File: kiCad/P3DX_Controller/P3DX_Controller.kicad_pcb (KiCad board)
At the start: 2 copper layers, 2 parts, among them U1 ESP32-WROOM-32E

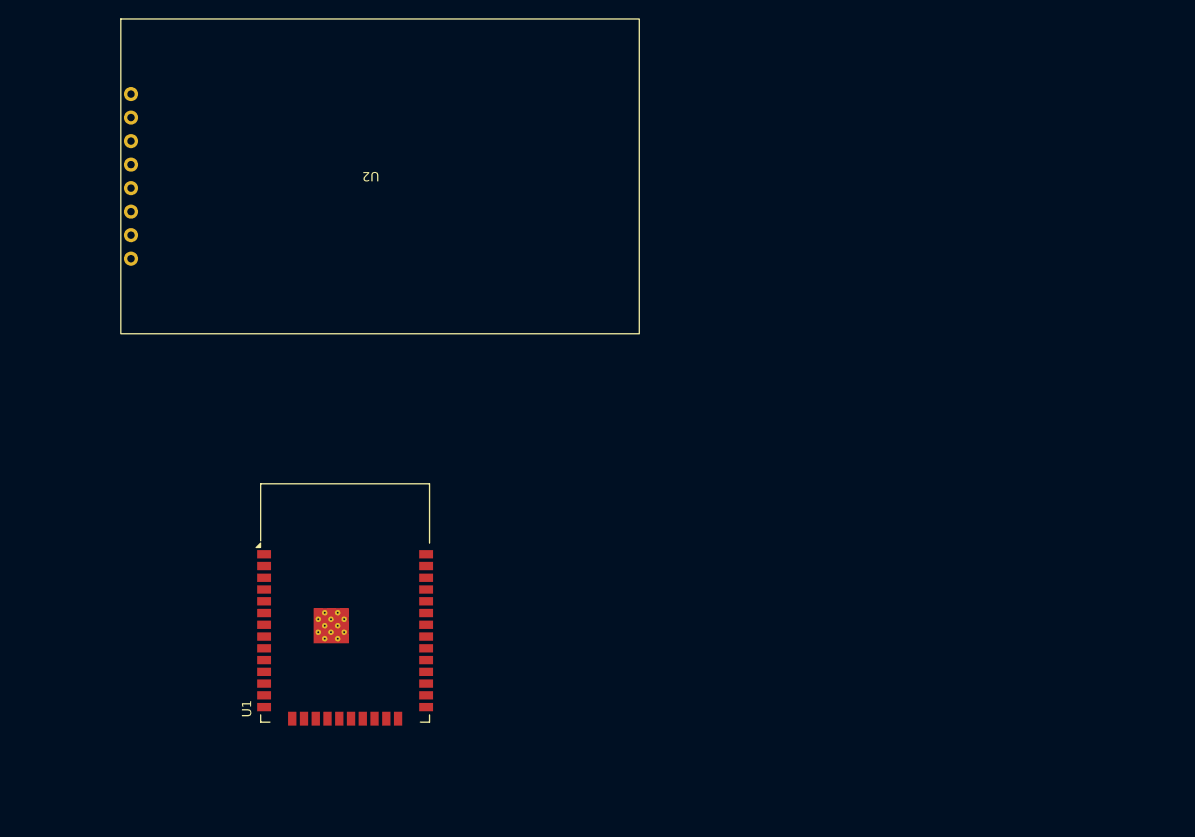
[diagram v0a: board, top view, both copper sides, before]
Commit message: 20251118
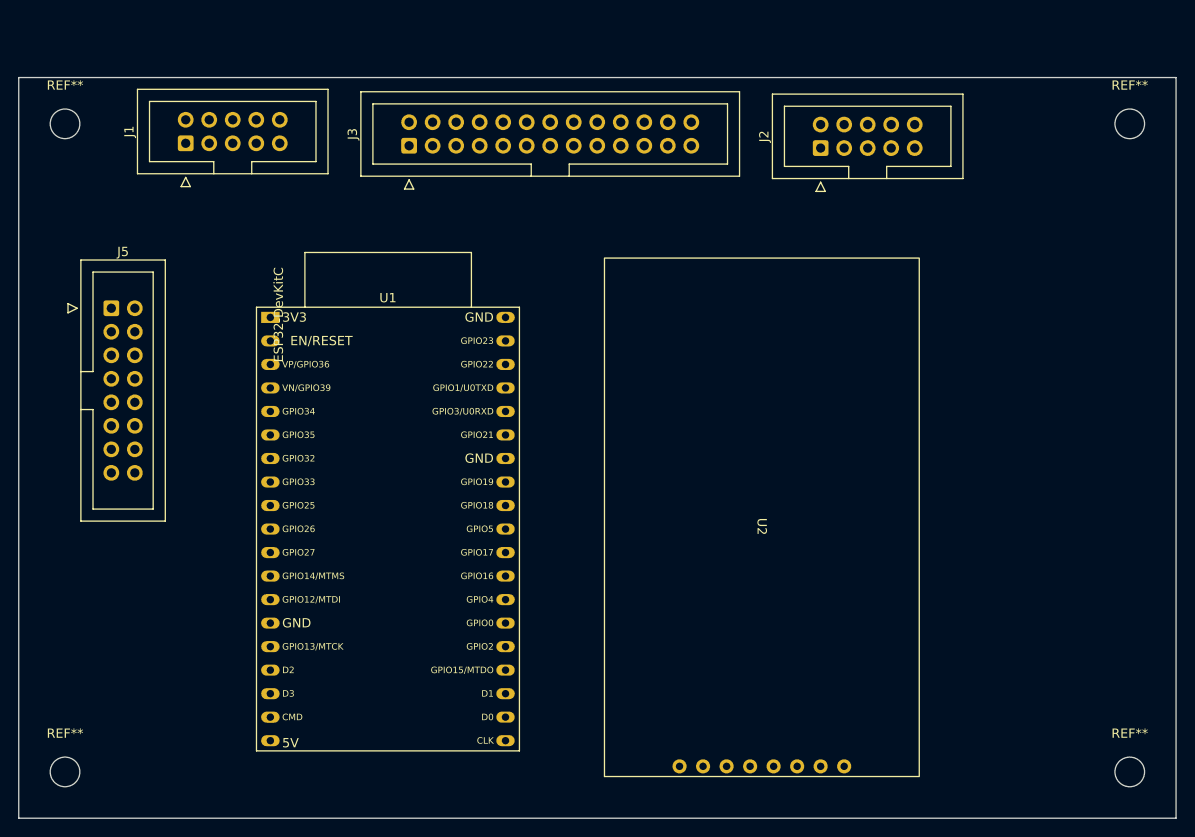
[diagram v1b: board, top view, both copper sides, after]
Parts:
- added J1: Conn_01x10_Pin, Connector_IDC:IDC-Header_2x05_P2.54mm_Vertical, F.Cu at (68.0, 57.1)
- added J2: Conn_01x10_Pin, Connector_IDC:IDC-Header_2x05_P2.54mm_Vertical, F.Cu at (136.6, 57.6)
- added J3: Conn_01x26_Pin, Connector_IDC:IDC-Header_2x13_P2.54mm_Vertical, F.Cu at (92.2, 57.4)
- added J5: Conn_01x16_Pin, Connector_IDC:IDC-Header_2x08_P2.54mm_Vertical, F.Cu at (60.0, 74.9)
- added REF**: MountingHole_3.2mm_M3, MountingHole:MountingHole_3.2mm_M3, F.Cu at (55.0, 55.0)
- added REF**: MountingHole_3.2mm_M3, MountingHole:MountingHole_3.2mm_M3, F.Cu at (55.0, 125.0)
- added REF**: MountingHole_3.2mm_M3, MountingHole:MountingHole_3.2mm_M3, F.Cu at (170.0, 55.0)
- added REF**: MountingHole_3.2mm_M3, MountingHole:MountingHole_3.2mm_M3, F.Cu at (170.0, 125.0)
- U1: value ESP32-WROOM-32E -> ESP32-DevKitC; footprint RF_Module:ESP32-WROOM-32D -> PCM_Espressif:ESP32-DevKitC
- moved U2 55.3 mm to (130.3, 97.5), turned to 90 degrees
- moved U1 34.8 mm to (77.2, 75.9)
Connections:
- U1 pad 1: Net-(U1-GND-Pad1) -> unconnected-(U1-3V3-Pad1)
- U1 pad 14: unconnected-(U1-IO12-Pad14) -> Net-(U1-GND-Pad14)
- U1 pad 15: Net-(U1-GND-Pad1) -> unconnected-(U1-MTCK/GPIO13/ADC2_CH4-Pad15)
- U1 pad 32: unconnected-(U1-NC-Pad32) -> Net-(U1-GND-Pad14)
- U1 pad 38: Net-(U1-GND-Pad1) -> Net-(U1-GND-Pad14)
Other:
- board outline added: 125 x 80 mm
